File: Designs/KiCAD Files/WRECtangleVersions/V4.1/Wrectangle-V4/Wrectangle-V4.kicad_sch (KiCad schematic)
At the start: 67 parts, among them J10 xBee-Antenna1, J2 USB_C_Receptacle_USB2.0_16P, J3 AnalogIn-Terminal3, J4 AnalogIn-Terminal2, J5 AnalogIn-Terminal1, J6 AnalogIn-Terminal0, J7 GPS-Antenna, J8 Micro_SD_Card, U1 STM32F405RGTx, U10 FT232RL, U11 BME280, U2 BNO085_C5189642, U3 MAX-M10S-00B, U4 H3LIS331DLTR, U9 XBP9X-DMUS-001

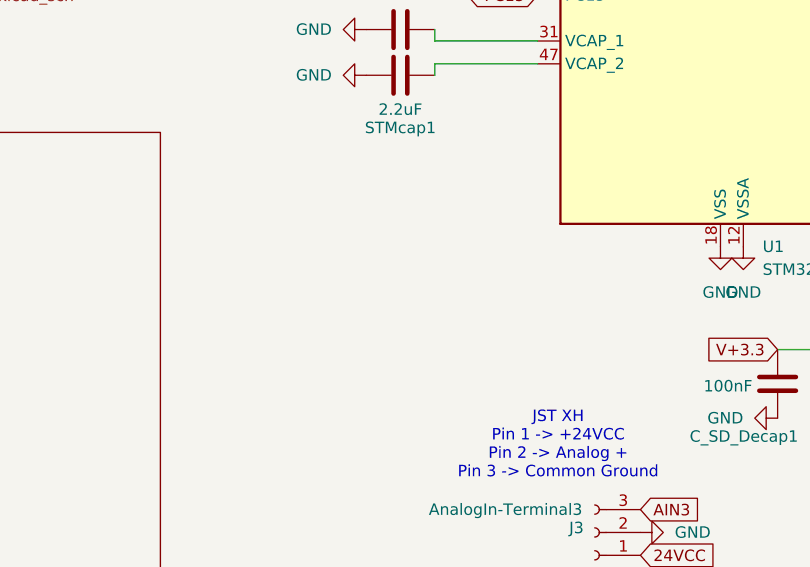
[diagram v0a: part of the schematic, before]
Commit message: h
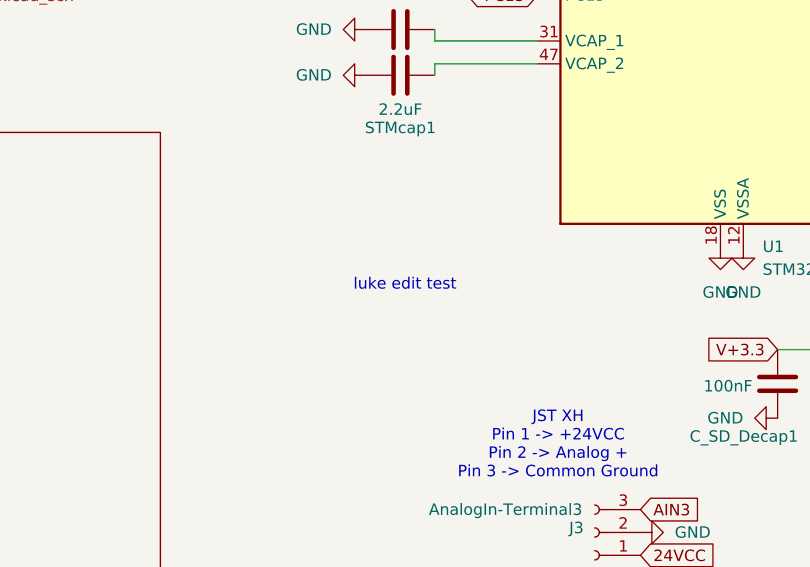
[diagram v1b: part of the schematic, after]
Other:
- note added: "luke edit test"
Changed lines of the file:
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@@
+		)
+	)
+	(text "luke edit test"
+		(exclude_from_sim no)
+		(at 24.638 130.048 0)
+		(effects
+			(font
+				(size 1.27 1.27)
+			)
 		)
 	)
